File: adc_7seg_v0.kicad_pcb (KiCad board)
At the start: 4 copper layers, 34 parts, among them J1 IN, J2 DC, Q1 BC847, U1 MC78M09C, U2 ICL7106, U3 TDSR1350, U4 TDSR1350, U5 TDSR1350

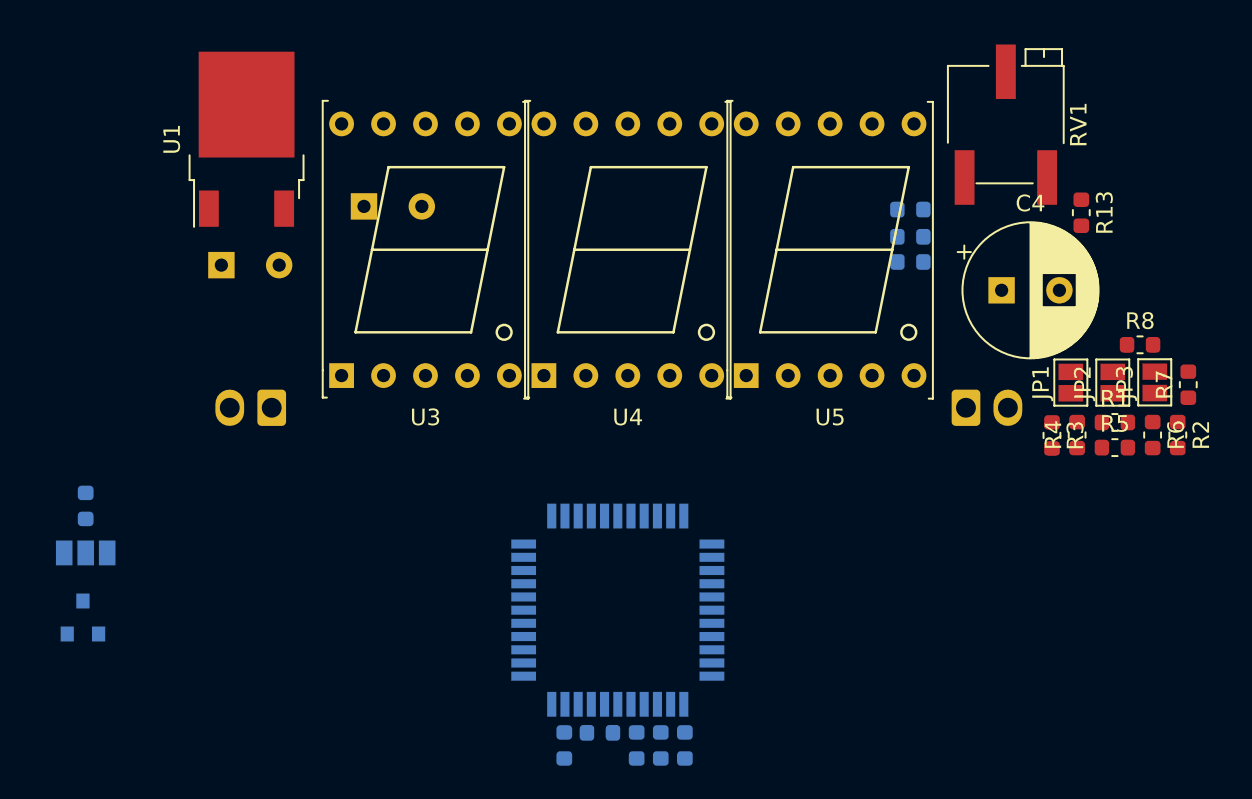
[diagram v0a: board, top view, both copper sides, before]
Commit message: second pokus of via, update gitignore
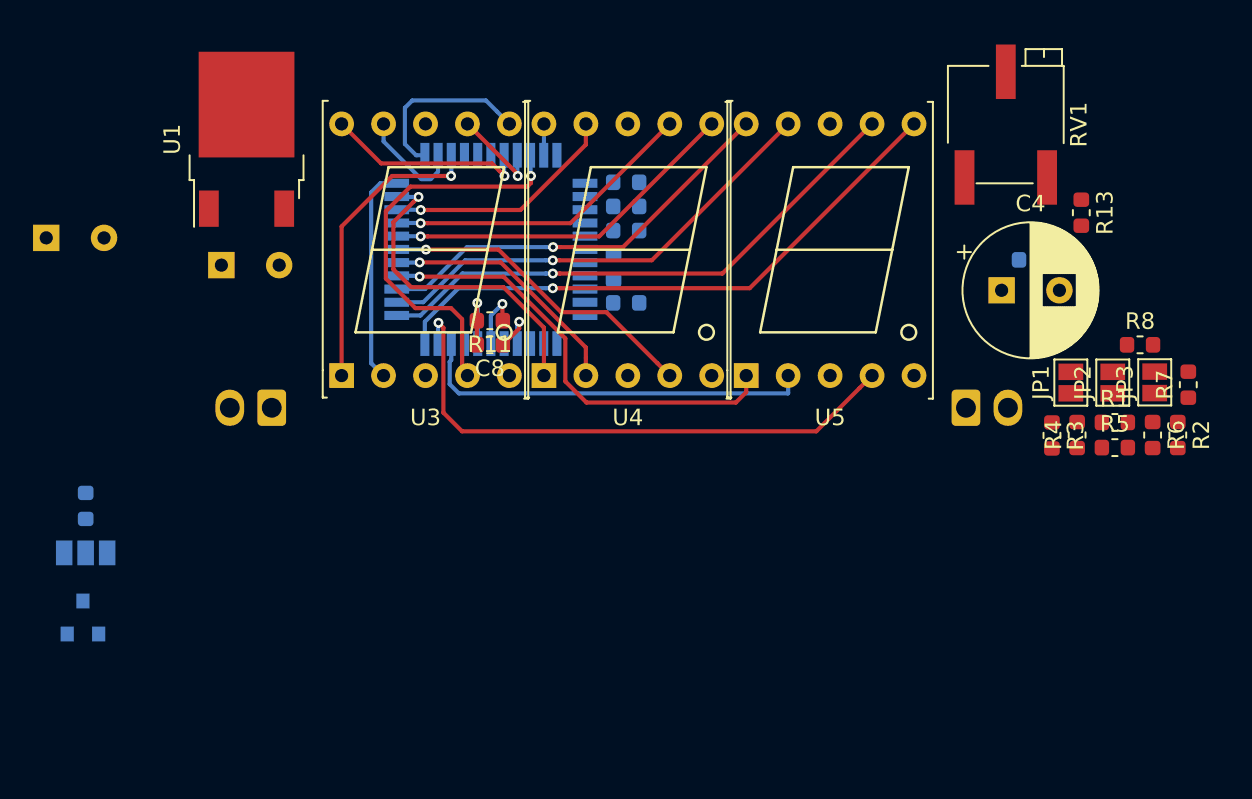
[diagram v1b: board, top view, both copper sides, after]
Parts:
- C8, R11: moved to F.Cu
- moved C7 34.3 mm to (193.2, 86.4), turned to 0 degrees
- moved R10 32.7 mm to (193.2, 87.9), turned to 0 degrees
- moved C6 31.2 mm to (193.2, 89.3), turned to 0 degrees
- moved C5 28.2 mm to (192.4, 91.6), turned to 90 degrees
- moved C9 27.1 mm to (193.2, 93.7), turned to 180 degrees
- moved R11 26.0 mm to (184.9, 94.8)
- moved C8 26.0 mm to (184.9, 96.3)
- moved U2 23.2 mm to (185.0, 90.5), turned to 90 degrees
- moved C2 19.3 mm to (158.1, 89.8)
- moved C3 7.97 mm to (217.7, 91.1)
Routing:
- net Net-(U2-Pad11): track 0.00 -> 35.9 mm, vias 0 -> 1
- net Net-(U2-Pad10): track 0.00 -> 34.7 mm, vias 0 -> 1
- net Net-(U2-Pad12): track 0.00 -> 33.6 mm, vias 0 -> 1
- net Net-(U2-Pad13): track 0.00 -> 28.2 mm, vias 0 -> 1
- net Net-(U2-Pad15): track 0.00 -> 27.1 mm, vias 0 -> 1
- net Net-(U2-Pad14): track 0.00 -> 25.3 mm, vias 0 -> 1
- net Net-(U2-Pad9): track 0.00 -> 24.3 mm
- net Net-(U2-Pad31): track 0.00 -> 24.0 mm, vias 0 -> 1
- net Net-(U2-Pad18): track 0.00 -> 21.9 mm, vias 0 -> 1
- net Net-(U2-Pad21): track 0.00 -> 19.8 mm, vias 0 -> 1
- net Net-(U2-Pad17): track 0.00 -> 19.7 mm, vias 0 -> 1
- net Net-(U2-Pad19): track 0.00 -> 19.0 mm, vias 0 -> 1
- net Net-(U2-Pad25): track 0.00 -> 18.2 mm, vias 0 -> 1
- net Net-(U2-Pad16): track 0.00 -> 15.3 mm, vias 0 -> 1
- net Net-(U2-Pad20): track 0.00 -> 14.3 mm, vias 0 -> 1
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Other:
- net class Default: trace_width 0.25 -> 0.254

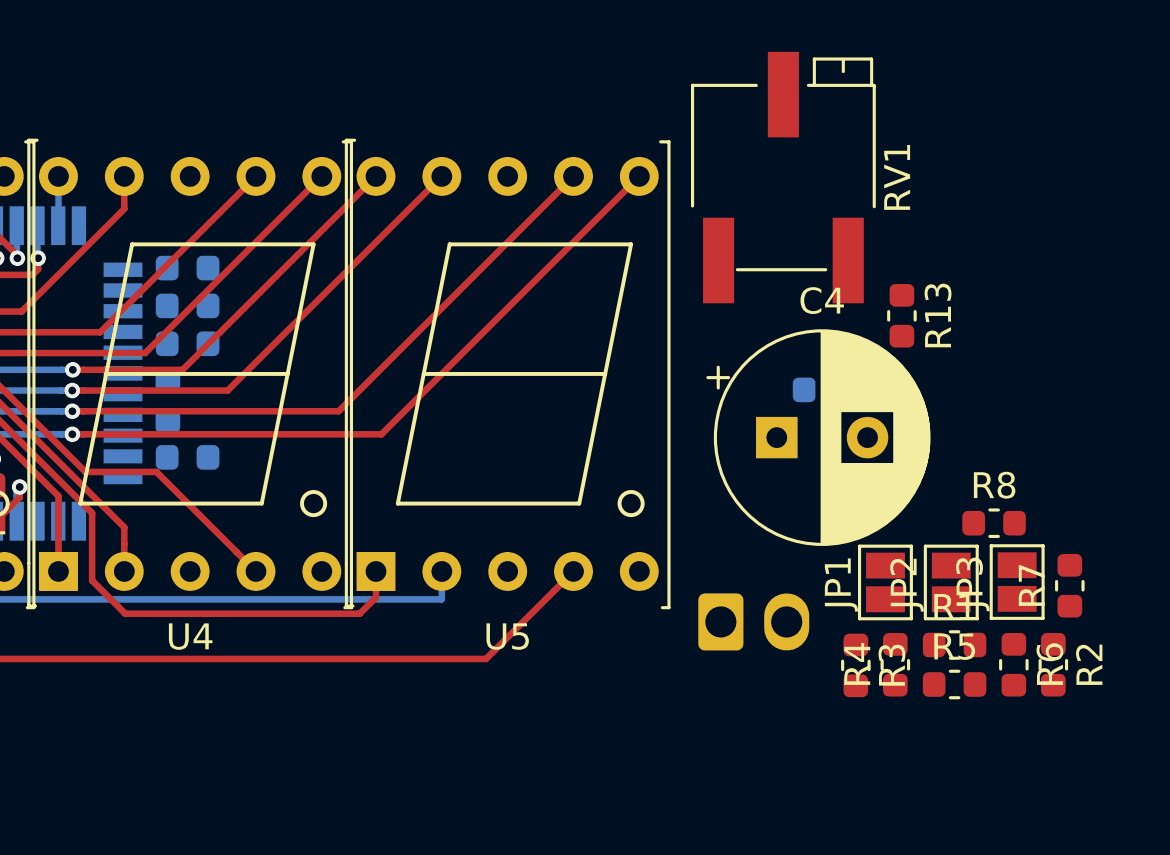
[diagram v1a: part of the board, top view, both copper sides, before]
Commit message: last wip back up
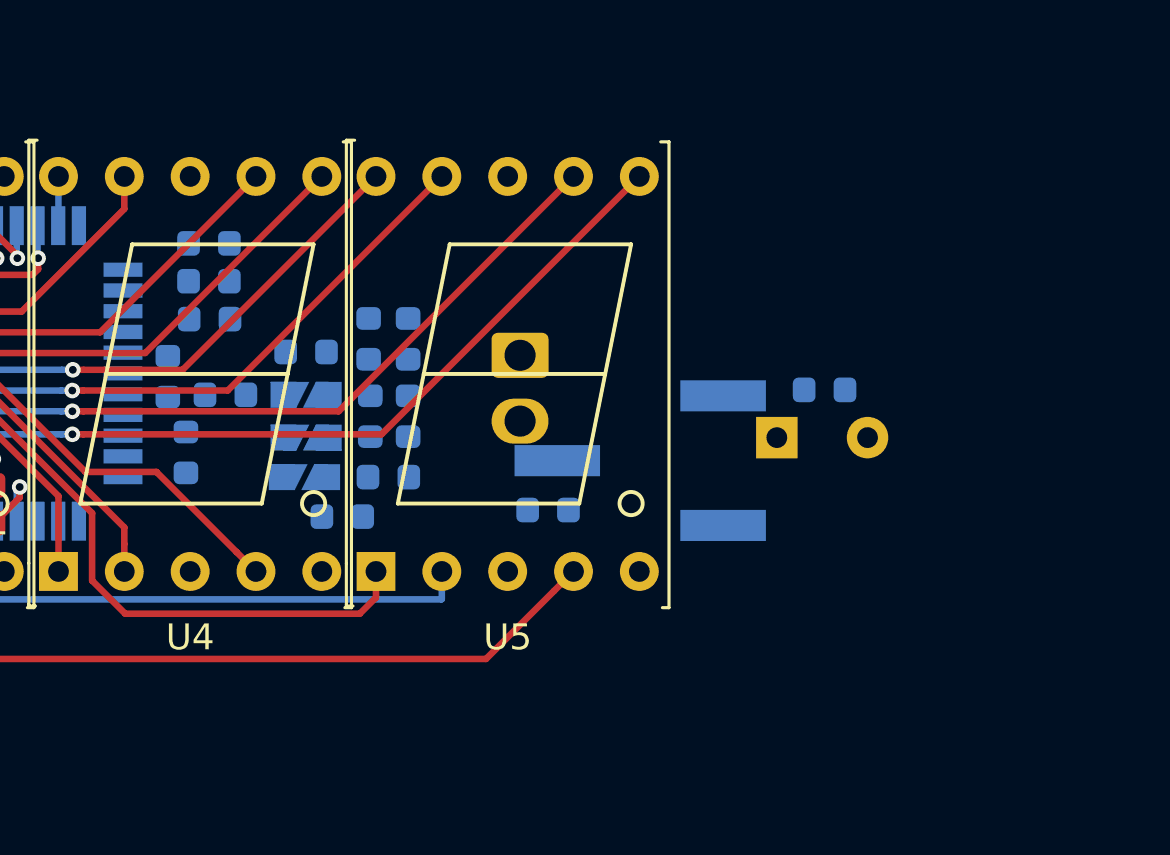
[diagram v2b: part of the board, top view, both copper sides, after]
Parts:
- C4, R1, R13, R2, R3, R4, R5, R6, R7, R8, RV1: moved to B.Cu
- JP1, JP2, JP3: footprint Jumper:SolderJumper-2_P1.3mm_Open_Pad1.0x1.5mm -> KLIB_Mechanical:Jumper; moved to B.Cu
- moved R7 30.8 mm to (197.7, 89.7), turned to 180 degrees
- moved R8 30.1 mm to (194.6, 91.3)
- moved JP3 28.4 mm to (197.7, 91.3), turned to 180 degrees
- moved R2 27.9 mm to (201.7, 89.2), turned to 90 degrees
- moved R6 27.9 mm to (200.2, 89.2), turned to 90 degrees
- moved JP2 25.5 mm to (197.7, 93.0), turned to 180 degrees
- moved R5 24.8 mm to (200.2, 92.1), turned to 90 degrees
- moved R1 22.9 mm to (201.7, 92.1), turned to 90 degrees
- moved JP1 22.8 mm to (197.7, 94.5), turned to 180 degrees
- moved R4 20.9 mm to (200.9, 94.5), turned to 0 degrees
- moved R3 20.6 mm to (199.1, 96.0), turned to 0 degrees
- moved R13 15.6 mm to (207.1, 95.8), turned to 180 degrees
- moved J1 12.9 mm to (206.0, 89.8), turned to 270 degrees
- moved RV1 12.2 mm to (210.6, 93.9), turned to 0 degrees
- moved C6 1.28 mm to (194.0, 88.4)
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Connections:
- U3 pad 8: Net-(U3-Pad8) -> (no net)
- U4 pad 8: Net-(U4-Pad8) -> (no net)
- U5 pad 5: Net-(U5-Pad5) -> (no net)
- U5 pad 8: Net-(U5-Pad8) -> (no net)

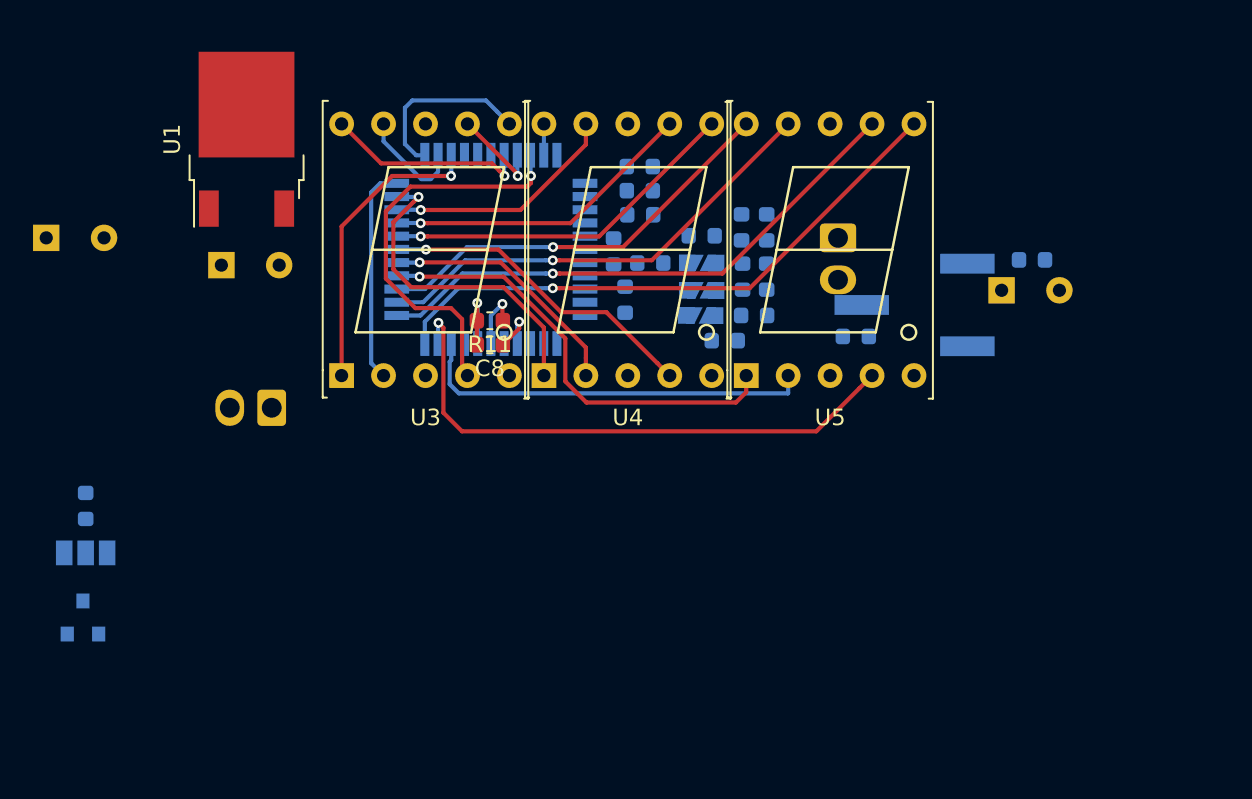
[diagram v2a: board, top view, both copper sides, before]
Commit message: last wip
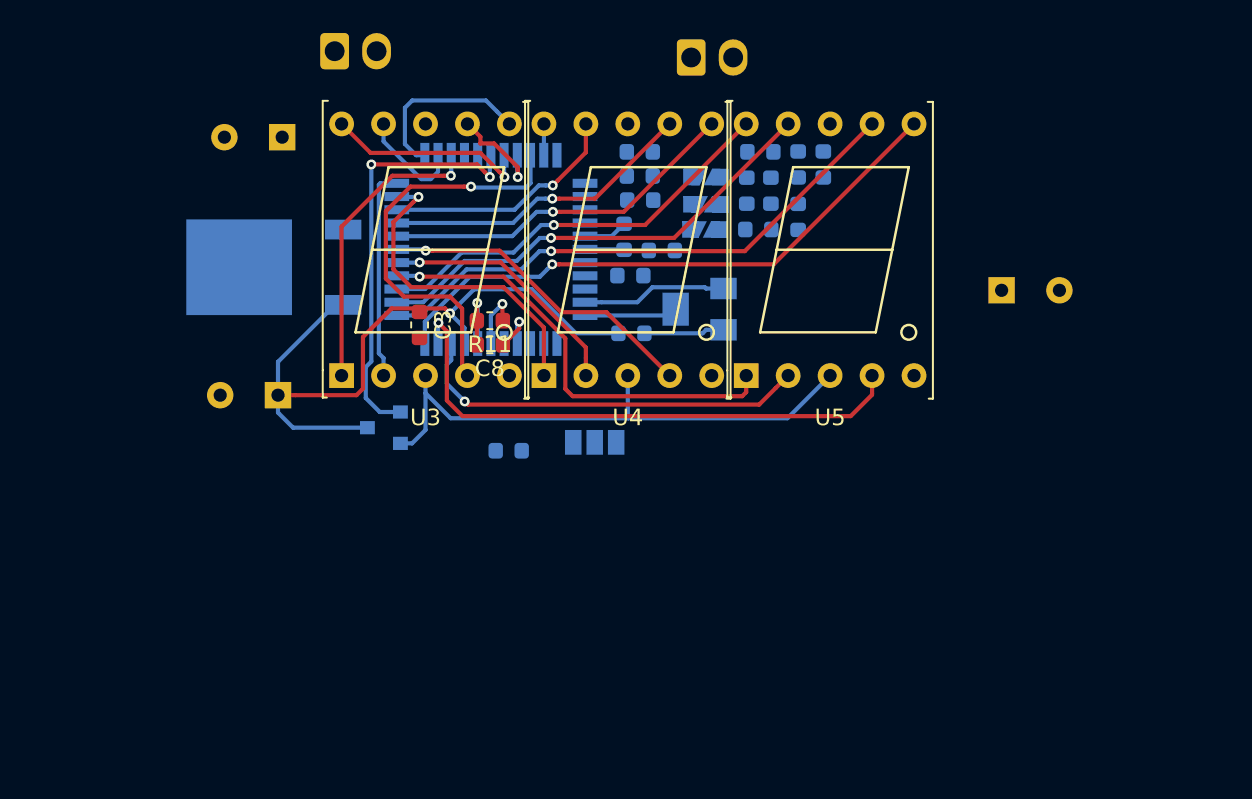
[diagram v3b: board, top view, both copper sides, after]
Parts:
- C3: moved to F.Cu
- RV1: footprint KLALIB_Potenciometer_SMD:Potentiometer_Bourns_3269P_Horizontal -> KLALIB_Potenciometer_SMD:Potentiometer_SRPASSIVES_1801
- U1: moved to B.Cu
- moved C3 37.3 mm to (180.7, 95.1), turned to 270 degrees
- moved JP4 31.5 mm to (191.3, 102.2)
- moved R12 25.8 mm to (186.1, 102.7), turned to 180 degrees
- moved J2 21.9 mm to (175.5, 78.5), turned to 0 degrees
- moved Q1 21.5 mm to (178.5, 101.3), turned to 180 degrees
- moved C2 17.0 mm to (172.1, 99.3), turned to 180 degrees
- moved J1 14.1 mm to (197.1, 78.9), turned to 0 degrees
- moved R13 13.6 mm to (193.5, 95.6)
- moved RV1 13.0 mm to (197.6, 94.1)
- moved C1 8.58 mm to (172.3, 83.7), turned to 180 degrees
- moved U1 7.92 mm to (171.8, 91.6), turned to 180 degrees
- moved R3 7.03 mm to (201.2, 89.3)
- moved R4 6.54 mm to (203.6, 88.5), turned to 90 degrees
- moved R6 6.25 mm to (205.1, 85.3)
- moved R7 6.20 mm to (201.3, 84.6)
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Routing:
- net +9V: track 0.00 -> 43.0 mm, vias 0 -> 1
- net Net-(Q1-Pad2): track 0.00 -> 33.9 mm
- net Net-(Q1-Pad1): track 0.00 -> 25.6 mm, vias 0 -> 2
- net Net-(C5-Pad2): track 0.00 -> 11.5 mm
- net Net-(RV1-Pad2): track 0.00 -> 5.64 mm
- net Net-(R13-Pad1): track 0.00 -> 4.84 mm
- net Net-(C5-Pad1): track 0.00 -> 2.38 mm
- net Net-(U2-Pad10): track 34.7 -> 34.0 mm
- net Net-(U2-Pad30): track 5.68 -> 6.29 mm
- net Net-(U2-Pad9): track 24.3 -> 24.5 mm, vias 0 -> 1

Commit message: almost last  version
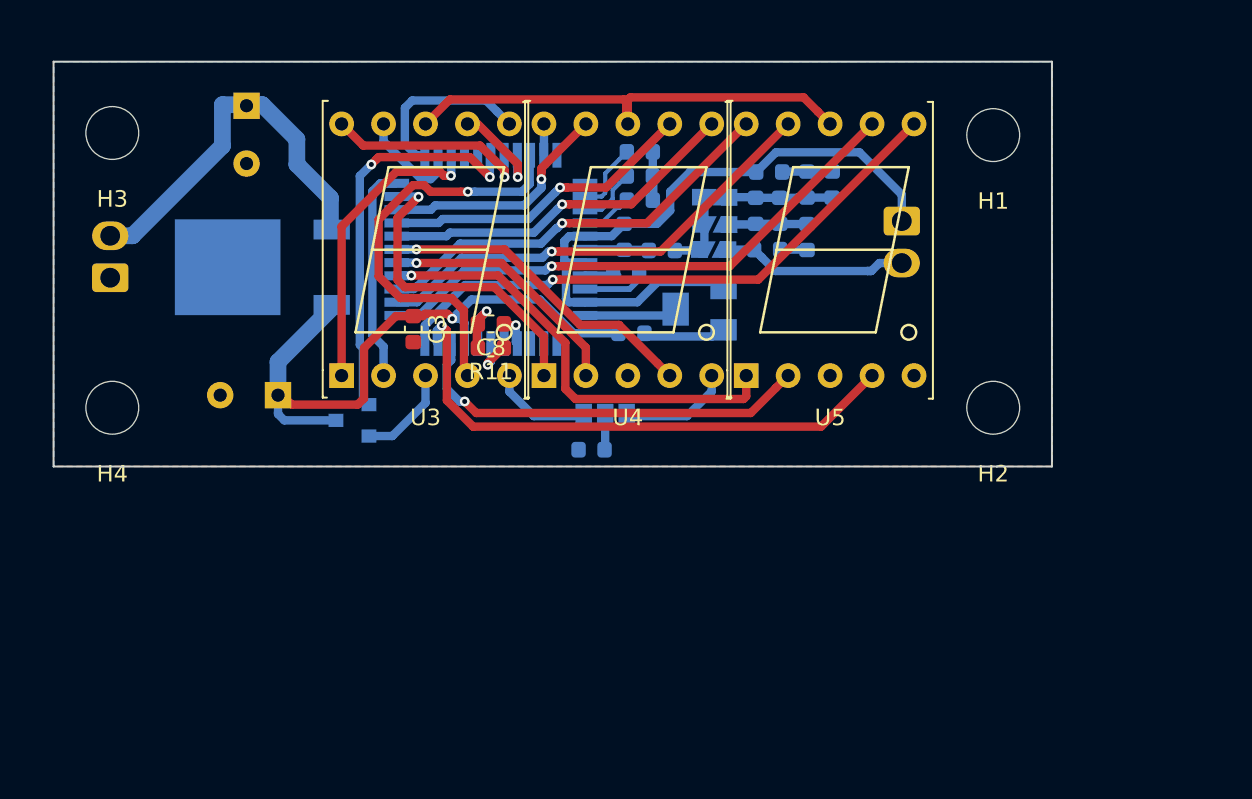
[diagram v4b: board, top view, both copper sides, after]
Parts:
- removed C4: 100u, Capacitor_THT:CP_Radial_D8.0mm_P3.50mm
- added H1: Bolt, KLALIB_Mechanical:Bolt_M3, F.Cu at (215.4, 83.6)
- added H2: Bolt, KLALIB_Mechanical:Bolt_M3, F.Cu at (215.4, 100.1)
- added H3: Bolt, KLALIB_Mechanical:Bolt_M3, F.Cu at (162.1, 83.4)
- added H4: Bolt, KLALIB_Mechanical:Bolt_M3, F.Cu at (162.1, 100.1)
- moved J2 19.3 mm to (161.9, 92.2), turned to 90 degrees
- moved J1 16.1 mm to (209.9, 88.8), turned to 270 degrees
- moved R12 5.02 mm to (191.1, 102.6)
- moved C1 2.88 mm to (170.2, 81.8), turned to 270 degrees
- moved Q1 1.96 mm to (176.6, 100.8)
- moved JP4 1.71 mm to (191.9, 100.6)
- moved R11 1.65 mm to (185.0, 96.5)
- moved JP1 1.33 mm to (198.5, 90.5)
- moved JP2 1.33 mm to (198.5, 89.0)
- moved JP3 1.33 mm to (198.5, 87.3)
- moved R1 1.33 mm to (202.5, 88.2)
- moved R2 1.33 mm to (204.1, 86.6)
- moved R3 1.33 mm to (201.7, 90.5)
- moved R4 1.33 mm to (204.1, 89.7)
- moved R5 1.33 mm to (201.0, 88.2)
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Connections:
- U3 pad 8: (no net) -> Net-(U3-Pad8)
- U4 pad 3: Net-(Q1-Pad2) -> (no net)
- U4 pad 8: (no net) -> Net-(U3-Pad8)
- U5 pad 3: Net-(Q1-Pad2) -> (no net)
- U5 pad 8: (no net) -> Net-(U3-Pad8)
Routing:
- net Net-(C5-Pad2): track 11.5 -> 41.0 mm
- net Net-(U3-Pad8): track 0.00 -> 28.6 mm
- net Net-(Q1-Pad2): track 33.9 -> 5.91 mm
- net Net-(C1-Pad1): track 0.00 -> 23.3 mm
- net Net-(J1-Pad2): track 0.00 -> 11.5 mm
- net Net-(JP3-Pad1): track 0.00 -> 7.08 mm
- net Net-(JP4-Pad3): track 0.00 -> 6.73 mm
- net Net-(JP4-Pad1): track 0.00 -> 6.09 mm
- net Net-(JP2-Pad1): track 0.00 -> 4.98 mm
- net Net-(JP1-Pad2): track 0.00 -> 4.95 mm
- net Net-(C7-Pad1): track 0.00 -> 4.34 mm
- net Net-(C9-Pad1): track 0.00 -> 3.78 mm
- net Net-(R10-Pad1): track 0.00 -> 3.68 mm
- net Net-(C6-Pad1): track 0.00 -> 3.13 mm
- net Net-(R2-Pad2): track 0.00 -> 3.03 mm
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- added copper zone on B.Cu, net GND
- added copper zone on F.Cu, net GND
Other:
- board outline added: 60.5 x 24.5 mm
- copper layers 4 -> 2
- net class Default: clearance 0.2 -> 0.1524
- rule trace_clearance: 0.2 -> 0.1524
